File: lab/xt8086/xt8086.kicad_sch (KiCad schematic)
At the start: 14 parts, among them J1 Ext Connector, U1 74LS04, U2 74LS74, U3 8086_Min_Mode, U4 WeAct RP2350B

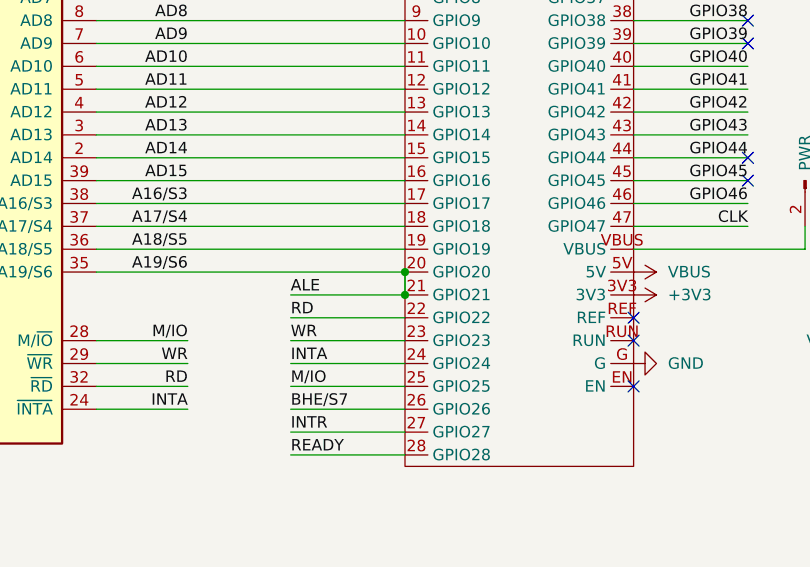
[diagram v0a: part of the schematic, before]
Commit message: LAB WIP
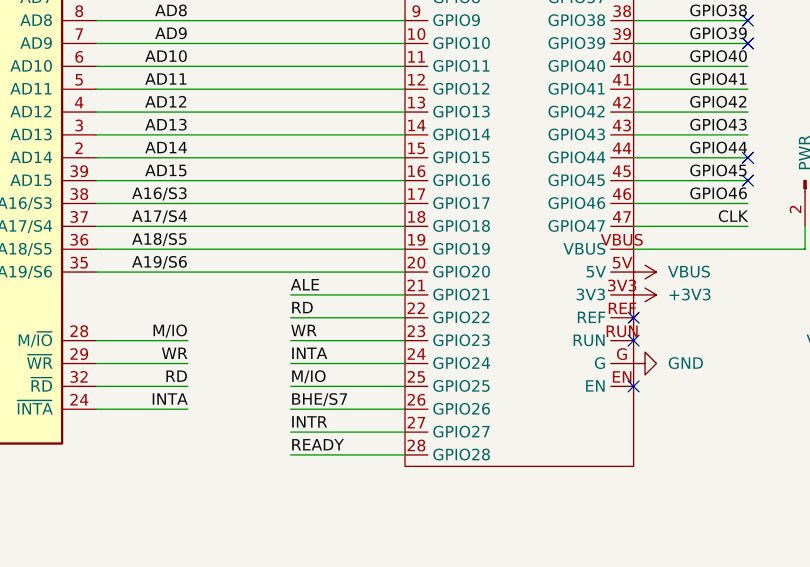
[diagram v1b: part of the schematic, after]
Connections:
- net A19/S6: no longer J1.23 (Pin_23), U3.25 (ALE), U4.21 (GPIO21)
- new net ALE: J1.23 (Pin_23), U3.25 (ALE), U4.21 (GPIO21)
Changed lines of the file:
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@@
-	)
-	(junction
-		(at 231.14 102.87)
-		(diameter 0)
-		(color 0 0 0 0)
 	)
 	(junction
@@
 	)
 	(junction
-		(at 231.14 100.33)
-		(diameter 0)
-		(color 0 0 0 0)
-	)
-	(junction
 		(at 26.67 144.78)
 		(diameter 0)
@@
 		)
 		(stroke
-			(width 0)
-			(type default)
-		)
-	)
-	(wire
-		(pts
-			(xy 231.14 100.33) (xy 231.14 102.87)
-		)
-		(stroke

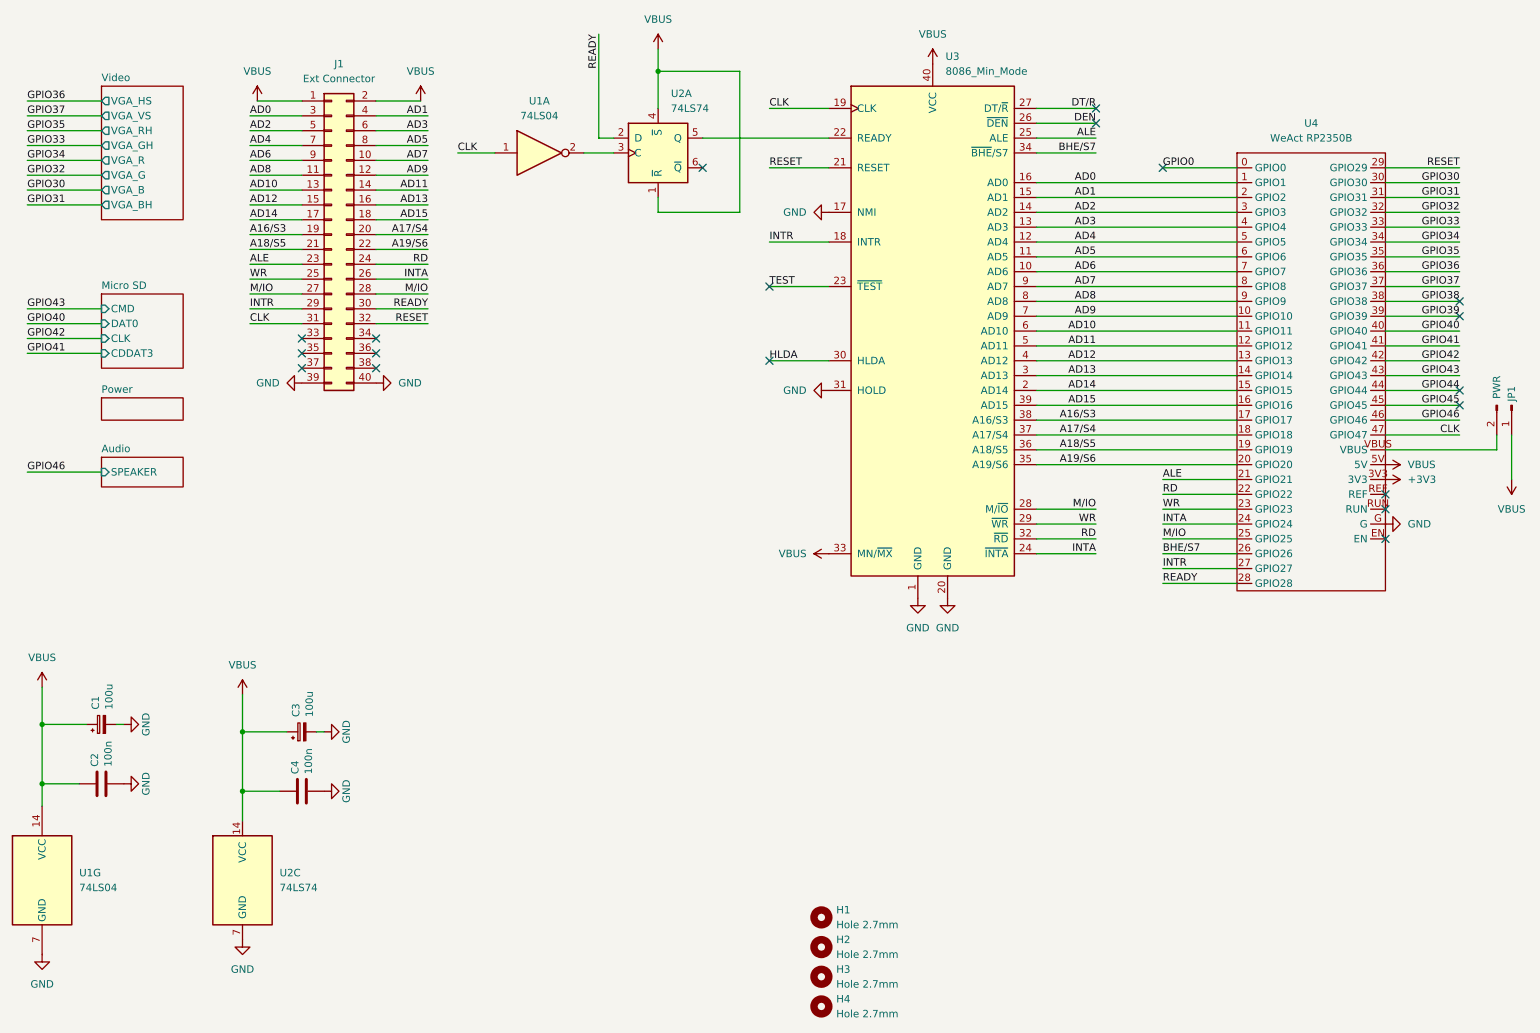
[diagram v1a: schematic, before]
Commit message: Board updates
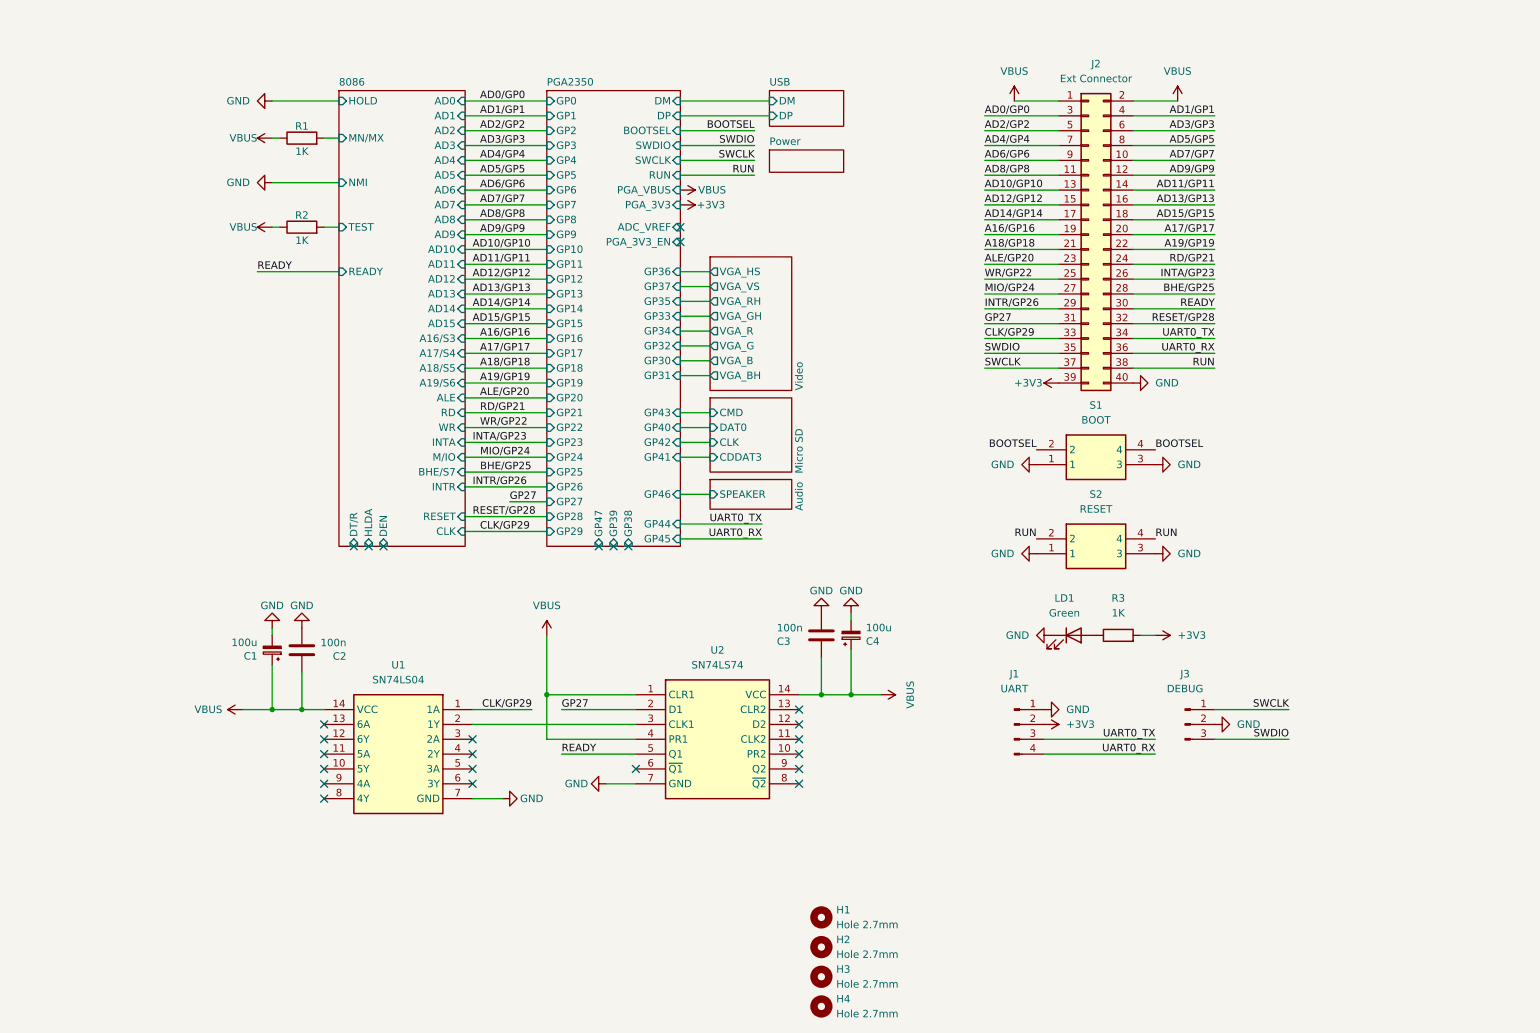
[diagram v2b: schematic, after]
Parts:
- removed C3: 100u, FRANK:CP_Elec_6.3x5.2, symbol Device:C_Polarized_Small
- removed C4: 100n, FRANK:C_0805_2012Metric, symbol Device:C
- removed JP1: PWR, FRANK:Jumper (solder), symbol Connector:Conn_01x02_Pin
- removed U1: 74LS04, FRANK:SOIC127P600X175-14N, symbol 74xx:74LS04
- removed U2: 74LS74, FRANK:SOIC127P600X175-14N, symbol 74xx:74LS74
- removed U3: 8086_Min_Mode, Package_DIP:DIP-40_W15.24mm, symbol MCU_Intel:8086_Min_Mode
- removed U4: WeAct RP2350B, FRANK:WeAct2350B, symbol FRANK:WeAct_2350B
- added C3: 100n, FRANK:C_0805_2012Metric, symbol Device:C
- added C4: 100u, Capacitor_THT:CP_Radial_D6.3mm_P2.50mm, symbol Device:C_Polarized_Small
- added J1: UART, FRANK:JST_SH_BM04B-SRSS-TB_1x04-1MP_P1.00mm_Vertical, symbol Connector:Conn_01x04_Pin
- added J3: DEBUG, FRANK:JST_SH_BM03B-SRSS-TB_1x03-1MP_P1.00mm_Vertical, symbol Connector:Conn_01x03_Pin
- added LD1: Green, FRANK:LED (0805), symbol Device:LED
- added R1, R2, R3: 1K, FRANK:R_0805_2012Metric, symbol Device:R
- added S1: BOOT, FRANK:KMR_2, symbol KMR221G_LFS:KMR221G_LFS
- added S2: RESET, FRANK:KMR_2, symbol KMR221G_LFS:KMR221G_LFS
- added U1: SN74LS04, FRANK:DIP14, symbol SN74LS04N:SN74LS04N
- added U2: SN74LS74, FRANK:DIP14, symbol SN74LS74ANE4:SN74LS74ANE4
- C1: footprint FRANK:CP_Elec_6.3x5.2 -> Capacitor_THT:CP_Radial_D6.3mm_P2.50mm
- renumbered J1 to J2
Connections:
- net +3V3: now also J2.39 (Pin_39), J1.2 (Pin_2), R3.2
- net GND: now also C3.2, C4.2, J1.1 (Pin_1), J3.2 (Pin_2), LD1.1 (K), S1.1, S1.3, S2.1, S2.3, U1.7 (GND), U2.7 (GND); no longer J2.39 (Pin_39)
- net READY: now also U2.5 (Q1)
- net VBUS: now also C3.1, C4.1, R1.1, R2.1, U1.14 (VCC), U2.1 (CLR1), U2.14 (VCC), U2.4 (PR1)
- net CLK/GP29: now reaches J2.33 (Pin_33)
- net CLK/GP29: now also U1.1 (1A)
- net UART0_TX: now reaches J2.34 (Pin_34)
- net UART0_TX: now also J1.3 (Pin_3)
- net SWDIO: now reaches J2.35 (Pin_35)
- net SWDIO: now also J3.3 (Pin_3)
- net UART0_RX: now reaches J2.36 (Pin_36)
- net UART0_RX: now also J1.4 (Pin_4)
- net SWCLK: now reaches J2.37 (Pin_37)
- net SWCLK: now also J3.1 (Pin_1)
- net RUN: now reaches J2.38 (Pin_38)
- net RUN: now also S2.2, S2.4
- net A16/S3 renamed A16/GP16
- net A17/S4 renamed A17/GP17
- net A18/S5 renamed A18/GP18
- net A19/S6 renamed A19/GP19
- net AD0 renamed AD0/GP0
- net AD1 renamed AD1/GP1
- net AD10 renamed AD10/GP10
- net AD11 renamed AD11/GP11
- net AD12 renamed AD12/GP12
- net AD13 renamed AD13/GP13
- net AD14 renamed AD14/GP14
- net AD15 renamed AD15/GP15
- net AD2 renamed AD2/GP2
- net AD3 renamed AD3/GP3
- net AD4 renamed AD4/GP4
- net AD5 renamed AD5/GP5
- net AD6 renamed AD6/GP6
- net AD7 renamed AD7/GP7
- net AD8 renamed AD8/GP8
- net AD9 renamed AD9/GP9
- net ALE renamed ALE/GP20
- net CLK renamed GP27
- net GP27: now also U2.2 (D1)
- net INTA renamed INTA/GP23
- net INTR renamed INTR/GP26
- net M/IO renamed BHE/GP25
- net BHE/GP25: no longer J2.27 (Pin_27)
- net RD renamed RD/GP21
- net RESET renamed RESET/GP28
- net WR renamed WR/GP22
- new net: LD1.2 (A), R3.1
- new net: U1.2 (1Y), U2.3 (CLK1)
- new net 8086/MN/MX: R1.2
- new net 8086/TEST: R2.2
- new net BOOTSEL: S1.2, S1.4
- new net MIO/GP24: J2.27 (Pin_27)
- no-connect marks 19 -> 25
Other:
- added sheet 8086 (8086.kicad_sch)
- added sheet PGA2350 (pga2350.kicad_sch)
- added sheet USB (usb.kicad_sch)
- moved on the sheet: J2

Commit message: xt8086 WIP
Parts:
- C1, C4: footprint Capacitor_THT:CP_Radial_D6.3mm_P2.50mm -> FRANK:CP_Radial_D6.3mm_P2.50mm
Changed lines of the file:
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@@
 			)
 		)
-		(property "Footprint" "Capacitor_THT:CP_Radial_D6.3mm_P2.50mm"
+		(property "Footprint" "FRANK:CP_Radial_D6.3mm_P2.50mm"
 			(at 66.04 132.08 0)
 			(effects
@@
 			)
 		)
-		(property "Footprint" "Capacitor_THT:CP_Radial_D6.3mm_P2.50mm"
+		(property "Footprint" "FRANK:CP_Radial_D6.3mm_P2.50mm"
 			(at 165.1 129.54 0)
 			(effects

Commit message: Boards WIP
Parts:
- C1, C4: footprint FRANK:CP_Radial_D6.3mm_P2.50mm -> xt8086:CP_Radial_D6.3mm_P2.50mm; symbol Device:C_Polarized_Small -> xt8086:C_Polarized_Small
- C2, C3: footprint FRANK:C_0805_2012Metric -> xt8086:C_0805_2012Metric; symbol Device:C -> xt8086:C
- H1, H2, H3, H4: footprint FRANK:Mounting Hole (2.7mm) -> xt8086:Mounting Hole (2.7mm); symbol Mechanical:MountingHole -> xt8086:MountingHole
- J1: footprint FRANK:JST_SH_BM04B-SRSS-TB_1x04-1MP_P1.00mm_Vertical -> xt8086:JST_SH_BM04B-SRSS-TB_1x04-1MP_P1.00mm_Vertical; symbol Connector:Conn_01x04_Pin -> xt8086:Conn_01x04_Pin
- J2: footprint FRANK:PinHeader_2x20_P2.54mm_Vertical -> xt8086:PinHeader_2x20_P2.54mm_Vertical; symbol Connector_Generic:Conn_02x20_Odd_Even -> xt8086:Conn_02x20_Odd_Even
- J3: footprint FRANK:JST_SH_BM03B-SRSS-TB_1x03-1MP_P1.00mm_Vertical -> xt8086:JST_SH_BM03B-SRSS-TB_1x03-1MP_P1.00mm_Vertical; symbol Connector:Conn_01x03_Pin -> xt8086:Conn_01x03_Pin
- LD1: footprint FRANK:LED (0805) -> xt8086:LED_0805_2012Metric_Pad1.15x1.40mm_HandSolder; symbol Device:LED -> xt8086:LED; KiLib_Generator (none) -> SMD_2terminal_chip_molded
- R1, R2, R3: footprint FRANK:R_0805_2012Metric -> xt8086:R_0805_2012Metric; symbol Device:R -> xt8086:R
- S1, S2: footprint FRANK:KMR_2 -> xt8086:KMR_2; symbol KMR221G_LFS:KMR221G_LFS -> xt8086:KMR221G_LFS
- U1: footprint FRANK:DIP14 -> xt8086:DIP14; symbol SN74LS04N:SN74LS04N -> xt8086:SN74LS04N
- U2: footprint FRANK:DIP14 -> xt8086:DIP14; symbol SN74LS74ANE4:SN74LS74ANE4 -> xt8086:SN74LS74ANE4
